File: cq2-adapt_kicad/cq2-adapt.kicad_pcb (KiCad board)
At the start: 2 copper layers, 9.2 x 6.7 mm, 10 parts

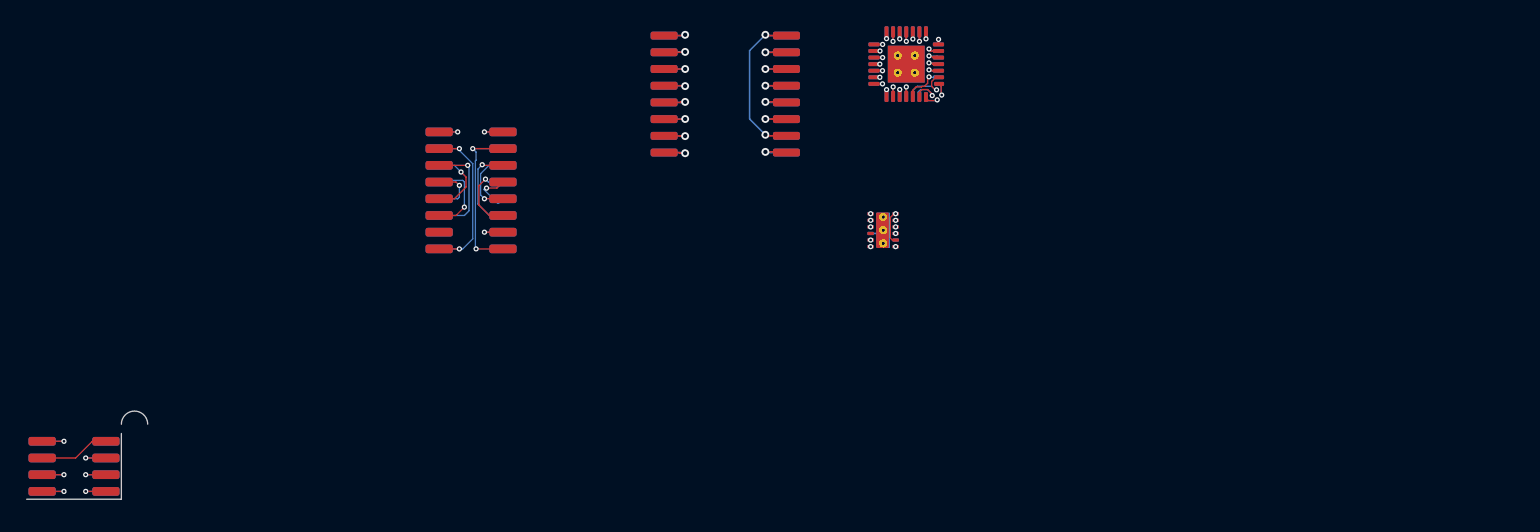
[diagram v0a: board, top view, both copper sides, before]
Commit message: CQ2 Adapter ordered
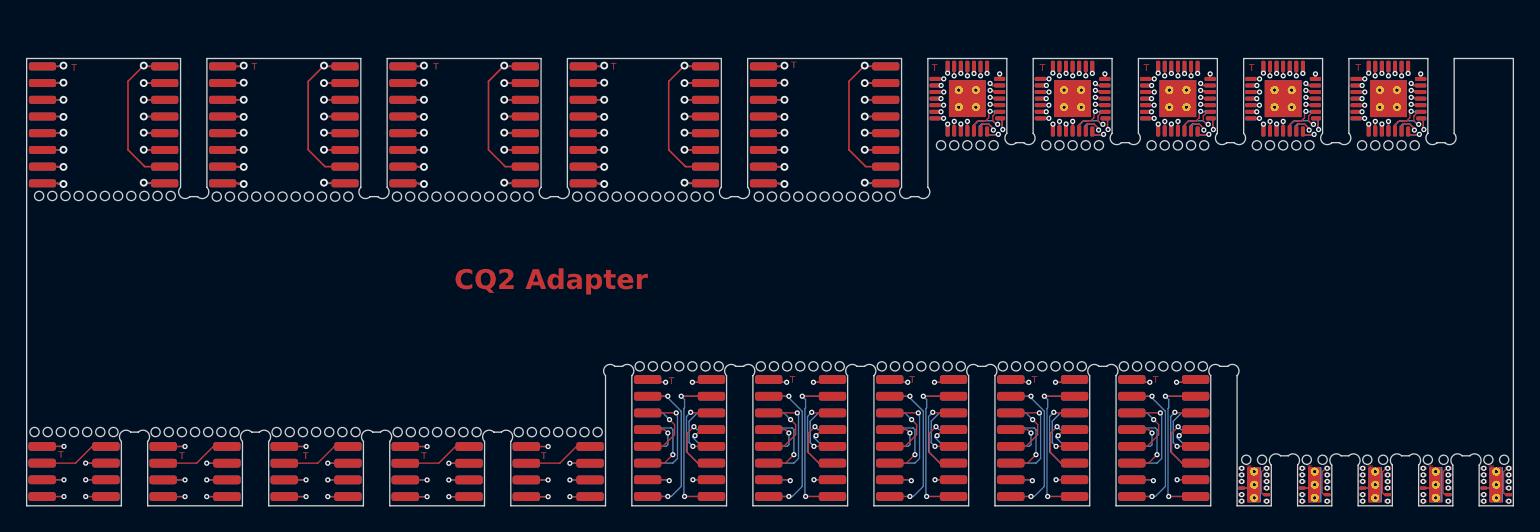
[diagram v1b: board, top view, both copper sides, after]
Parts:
- added ?: , , F.Cu at (85.9, 107.4)
- added ?: , , F.Cu at (85.3, 89.5)
- added ?: , , F.Cu at (89.9, 107.4)
- added ?: , , F.Cu at (108.3, 107.4)
- added ?: , , F.Cu at (143.1, 102.4)
- added ?: , , F.Cu at (103.3, 107.4)
- added ?: , , F.Cu at (177.2, 109.5)
- added ?: , , F.Cu at (125.5, 89.5)
- added ?: , , F.Cu at (171.4, 109.5)
- added ?: , , F.Cu at (149.3, 102.4)
- added ?: , , F.Cu at (114.8, 89.5)
- added ?: , , F.Cu at (87.9, 107.4)
- added ?: , , F.Cu at (115.5, 102.4)
- added ?: , , F.Cu at (125.7, 102.4)
- added ?: , , F.Cu at (146.4, 85.6)
- added ?: , , F.Cu at (135.9, 102.4)
- added ?: , , F.Cu at (106.8, 89.5)
- added ?: , , F.Cu at (96.0, 89.5)
- added ?: , , F.Cu at (129.6, 89.5)
- added ?: , , F.Cu at (84.3, 89.5)
- added ?: , , F.Cu at (123.7, 102.4)
- added ?: , , F.Cu at (102.3, 107.4)
- added ?: , , F.Cu at (66.8, 89.5)
- added ?: , , F.Cu at (88.3, 89.5)
- added ?: , , F.Cu at (145.4, 85.6)
- added ?: , , F.Cu at (139.1, 102.4)
- added ?: , , F.Cu at (123.5, 89.5)
- added ?: , , F.Cu at (113.8, 89.5)
- added ?: , , F.Cu at (134.9, 102.4)
- added ?: , , F.Cu at (167.4, 85.6)
- added ?: , , F.Cu at (70.5, 107.4)
- added ?: , , F.Cu at (166.8, 109.5)
- added ?: , , F.Cu at (82.3, 89.5)
- added ?: , , F.Cu at (101.0, 89.5)
- added ?: , , F.Cu at (104.3, 107.4)
- added ?: , , F.Cu at (166.4, 85.6)
- added ?: , , F.Cu at (80.7, 107.4)
- added ?: , , F.Cu at (153.4, 85.6)
- added ?: , , F.Cu at (99.1, 107.4)
- added ?: , , F.Cu at (96.1, 107.4)
- added ?: , , F.Cu at (117.5, 102.4)
- added ?: , , F.Cu at (122.5, 89.5)
- added ?: , , F.Cu at (127.5, 89.5)
- added ?: , , F.Cu at (78.7, 107.4)
- added ?: , , F.Cu at (138.4, 85.6)
- added ?: , , F.Cu at (94.0, 89.5)
- added ?: , , F.Cu at (98.0, 89.5)
- added ?: , , F.Cu at (93.0, 89.5)
- added ?: , , F.Cu at (144.4, 85.6)
- added ?: , , F.Cu at (88.9, 107.4)
- added ?: , , F.Cu at (157.6, 109.5)
- added ?: , , F.Cu at (95.1, 107.4)
- added ?: , , F.Cu at (65.8, 89.5)
- added ?: , , F.Cu at (98.1, 107.4)
- added ?: , , F.Cu at (95.0, 89.5)
- added ?: , , F.Cu at (72.8, 89.5)
- added ?: , , F.Cu at (69.5, 107.4)
- added ?: , , F.Cu at (87.3, 89.5)
- added ?: , , F.Cu at (120.7, 102.4)
- added ?: , , F.Cu at (160.4, 85.6)
- added ?: , , F.Cu at (170.4, 85.6)
- added ?: , , F.Cu at (114.5, 102.4)
- added ?: , , F.Cu at (111.8, 89.5)
- added ?: , , F.Cu at (126.7, 102.4)
- added ?: , , F.Cu at (107.8, 89.5)
- added ?: , , F.Cu at (76.7, 107.4)
- added ?: , , F.Cu at (140.1, 102.4)
- added ?: , , F.Cu at (110.8, 89.5)
- added ?: , , F.Cu at (168.0, 109.5)
- added ?: , , F.Cu at (122.7, 102.4)
- added ?: , , F.Cu at (131.9, 102.4)
- added ?: , , F.Cu at (161.4, 85.6)
- added ?: , , F.Cu at (137.4, 85.6)
- added ?: , , F.Cu at (172.6, 109.5)
- added ?: , , F.Cu at (120.5, 89.5)
- added ?: , , F.Cu at (163.4, 109.5)
- added ?: , , F.Cu at (121.5, 89.5)
- added ?: , , F.Cu at (126.5, 89.5)
- added ?: , , F.Cu at (80.3, 89.5)
- added ?: , , F.Cu at (111.5, 102.4)
- added ?: , , F.Cu at (136.4, 85.6)
- added ?: , , F.Cu at (107.3, 107.4)
- added ?: , , F.Cu at (115.8, 89.5)
- added ?: , , F.Cu at (112.5, 102.4)
- added ?: , , F.Cu at (130.6, 89.5)
- added ?: , , F.Cu at (69.8, 89.5)
- added ?: , , F.Cu at (113.5, 102.4)
- added ?: , , F.Cu at (74.8, 89.5)
- added ?: , , F.Cu at (67.8, 89.5)
- added ?: , , F.Cu at (129.9, 102.4)
- added ?: , , F.Cu at (153.3, 102.4)
- added ?: , , F.Cu at (145.1, 102.4)
- added ?: , , F.Cu at (130.9, 102.4)
- added ?: , , F.Cu at (65.5, 107.4)
- added ?: , , F.Cu at (73.8, 89.5)
- added ?: , , F.Cu at (142.1, 102.4)
- added ?: , , F.Cu at (83.3, 89.5)
- added ?: , , F.Cu at (158.4, 85.6)
- added ?: , , F.Cu at (154.4, 85.6)
- added ?: , , F.Cu at (133.9, 102.4)
- added ?: , , F.Cu at (75.7, 107.4)
- added ?: , , F.Cu at (148.3, 102.4)
- added ?: , , F.Cu at (105.3, 107.4)
- added ?: , , F.Cu at (66.5, 107.4)
- added ?: , , F.Cu at (68.5, 107.4)
- added ?: , , F.Cu at (102.0, 89.5)
- added ?: , , F.Cu at (142.4, 85.6)
- added ?: , , F.Cu at (116.8, 89.5)
- added ?: , , F.Cu at (124.7, 102.4)
- added ?: , , F.Cu at (176.0, 109.5)
- added ?: , , F.Cu at (159.4, 85.6)
- added ?: , , F.Cu at (134.4, 85.6)
- added ?: , , F.Cu at (77.7, 107.4)
- added ?: , , F.Cu at (71.5, 107.4)
- added ?: , , F.Cu at (103.0, 89.5)
- added ?: , , F.Cu at (141.1, 102.4)
- added ?: , , F.Cu at (132.9, 102.4)
- added ?: , , F.Cu at (70.8, 89.5)
- added ?: , , F.Cu at (100.0, 89.5)
- added ?: , , F.Cu at (162.4, 85.6)
- added ?: , , F.Cu at (93.1, 107.4)
- added ?: , , F.Cu at (152.3, 102.4)
- added ?: , , F.Cu at (86.9, 107.4)
- added ?: , , F.Cu at (86.3, 89.5)
- added ?: , , F.Cu at (154.3, 102.4)
- added ?: , , F.Cu at (79.3, 89.5)
- added ?: , , F.Cu at (168.4, 85.6)
- added ?: , , F.Cu at (75.8, 89.5)
- added ?: , , F.Cu at (150.3, 102.4)
- added ?: , , F.Cu at (151.4, 85.6)
- added ?: , , F.Cu at (97.0, 89.5)
- added ?: , , F.Cu at (144.1, 102.4)
- added ?: , , F.Cu at (162.2, 109.5)
- added ?: , , F.Cu at (67.5, 107.4)
- added ?: , , F.Cu at (152.4, 85.6)
- added ?: , , F.Cu at (124.5, 89.5)
- added ?: , , F.Cu at (169.4, 85.6)
- added ?: , , F.Cu at (99.0, 89.5)
- added ?: , , F.Cu at (68.8, 89.5)
- added ?: , , F.Cu at (121.7, 102.4)
- added ?: , , F.Cu at (89.3, 89.5)
- added ?: , , F.Cu at (106.3, 107.4)
- added ?: , , F.Cu at (83.9, 107.4)
- added ?: , , F.Cu at (74.7, 107.4)
- added ?: , , F.Cu at (158.8, 109.5)
- added ?: , , F.Cu at (79.7, 107.4)
- added ?: , , F.Cu at (109.8, 89.5)
- added ?: , , F.Cu at (135.4, 85.6)
- added ?: , , F.Cu at (128.6, 89.5)
- added ?: , , F.Cu at (151.3, 102.4)
- added ?: , , F.Cu at (108.8, 89.5)
- added ?: , , F.Cu at (94.1, 107.4)
- added ?: , , F.Cu at (143.4, 85.6)
- added ?: , , F.Cu at (81.3, 89.5)
- added ?: , , F.Cu at (97.1, 107.4)
- added ?: , , F.Cu at (150.4, 85.6)
- added ?: , , F.Cu at (71.8, 89.5)
- added ?: , , F.Cu at (112.8, 89.5)
- added ?: , , F.Cu at (116.5, 102.4)
- added ?: , , F.Cu at (84.9, 107.4)
- added UB1, UT1: 100 Mb/s, 0-standard:SOIC-16W, F.Cu at (125.5, 84.0)
- added UB1, UT1: 100 Mb/s, 0-standard:SOIC-16W, F.Cu at (98.2, 84.0)
- added UB1, UT1: 100 Mb/s, 0-standard:SOIC-16W, F.Cu at (111.8, 84.0)
- added UB1, UT1: 100 Mb/s, 0-standard:SOIC-16W, F.Cu at (84.5, 84.0)
- added UB2, UT2: LM27762, 1-special:integrated-144, F.Cu at (176.6, 111.4)
- added UB2, UT2: LM27762, 1-special:integrated-144, F.Cu at (167.4, 111.4)
- added UB2, UT2: LM27762, 1-special:integrated-144, F.Cu at (172.0, 111.4)
- added UB2, UT2: LM27762, 1-special:integrated-144, F.Cu at (162.8, 111.4)
- added UB3, UT3: LM5046MH, 1-special:integrated-129, F.Cu at (160.4, 82.1)
- added UB3, UT3: LM5046MH, 1-special:integrated-129, F.Cu at (168.4, 82.1)
- added UB3, UT3: LM5046MH, 1-special:integrated-129, F.Cu at (144.4, 82.0)
- added UB3, UT3: LM5046MH, 1-special:integrated-129, F.Cu at (152.4, 82.1)
- added UB4, UT4: 150 Mb/s, 0-standard:SOIC-16, F.Cu at (142.1, 107.8)
- added UB4, UT4: 150 Mb/s, 0-standard:SOIC-16, F.Cu at (151.3, 107.8)
- added UB4, UT4: 150 Mb/s, 0-standard:SOIC-16, F.Cu at (132.9, 107.8)
- added UB4, UT4: 150 Mb/s, 0-standard:SOIC-16, F.Cu at (123.7, 107.8)
- added UT5, UTB6: THVD1420, 0-standard:SOIC-8, F.Cu at (96.1, 110.4)
- added UT5, UTB6: THVD1420, 0-standard:SOIC-8, F.Cu at (105.3, 110.4)
- added UT5, UTB6: THVD1420, 0-standard:SOIC-8, F.Cu at (77.7, 110.4)
- added UT5, UTB6: THVD1420, 0-standard:SOIC-8, F.Cu at (86.9, 110.4)
- moved UB1 47.3 mm to (70.8, 84.0)
- moved UT1 47.3 mm to (70.8, 84.0)
- moved UB2 34.2 mm to (158.2, 111.4)
- moved UT2 34.2 mm to (158.2, 111.4)
- moved UB4 24.6 mm to (114.5, 107.8)
- moved UT4 24.6 mm to (114.5, 107.8)
- moved UB3 5.33 mm to (136.4, 82.0)
- moved UT3 5.33 mm to (136.4, 82.0)
- moved UT5 0.39 mm to (68.5, 110.4)
- moved UTB6 0.39 mm to (68.5, 110.4)
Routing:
- net Net-(UB4-GND2-Pad15): track 14.4 -> 82.3 mm, vias 2 -> 10
- net Net-(UB4-GND1-Pad2): track 14.8 -> 73.8 mm, vias 2 -> 10
- net Net-(UB1-VISO): track 13.5 -> 67.4 mm, vias 2 -> 5
- net Net-(UB4-A4): track 8.08 -> 40.4 mm, vias 1 -> 5
- net Net-(UB4-B4): track 6.98 -> 34.9 mm, vias 1 -> 5
- net Net-(UB4-A2): track 6.11 -> 30.5 mm, vias 1 -> 5
- net Net-(UB4-B2): track 5.76 -> 28.8 mm, vias 1 -> 5
- net Net-(UB4-A1): track 5.59 -> 27.9 mm, vias 1 -> 5
- net Net-(UB4-B1): track 5.40 -> 27.0 mm, vias 1 -> 5
- net Net-(UT5-VCC): track 5.38 -> 26.9 mm
- net Net-(UB4-EN1): track 0.00 -> 16.7 mm, vias 0 -> 5
- net Net-(UB4-A3): track 4.12 -> 20.6 mm, vias 1 -> 5
- net Net-(UB3-HS2): track 4.04 -> 20.2 mm, vias 1 -> 5
- net Net-(UB3-HO2): track 3.37 -> 16.9 mm, vias 1 -> 5
- net Net-(UB4-B3): track 3.69 -> 17.1 mm, vias 1 -> 5
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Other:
- board size 9.2 x 6.7 mm -> 113 x 34 mm
- board text added: "CQ2 Adapter"
- board text added: "T"
